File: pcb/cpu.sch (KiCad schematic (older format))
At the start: 28 parts, among them J100 Conn_02x05_Odd_Even, J101 Conn_02x05_Odd_Even, J102 Conn_02x05_Odd_Even, U100 MCIMX7S5EVM08SC, Y100 24MHz, Y101 32.768kHz

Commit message: pcb: remap schematic symbols
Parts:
- C100, C101, C102, C103, C104, C107, C108, C110: symbol pcb-rescue:C-Device-pcb-rescue -> Device:C
- D100: symbol pcb-rescue:D_Schottky-Device-pcb-rescue -> Device:D_Schottky
- J100, J101: symbol pcb-rescue:Conn_02x05_Odd_Even-Connector_Generic-pcb-rescue -> Connector_Generic:Conn_02x05_Odd_Even
- J102: symbol pcb-rescue:Conn_01x06-Connector_Generic-pcb-rescue -> Connector_Generic:Conn_01x06
- R102, R103, R104, R105, R106, R107, R108, R109, R110, R111: symbol pcb-rescue:R-Device-pcb-rescue -> Device:R
- RN100, RN101, RN102: symbol pcb-rescue:R_Pack04-Device-pcb-rescue -> Device:R_Pack04
- Y100: symbol pcb-rescue:Crystal_GND24-Device-pcb-rescue -> Device:Crystal_GND24
- Y101: symbol pcb-rescue:Crystal-Device-pcb-rescue -> Device:Crystal
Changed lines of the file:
@@
 	1700 1550 1900 1550
 $Comp
-L pcb-rescue:GND-power-pcb-rescue #PWR0101
+L power:GND #PWR0101
 U 1 1 5D1AEC8A
 P 1800 2050
@@
 	1900 2050 1800 2050
 $Comp
-L pcb-rescue:GND-power-pcb-rescue #PWR0102
+L power:GND #PWR0102
 U 1 1 5D1B0DA3
 P 3600 2950
@@
 NoConn ~ 3500 2350
 $Comp
-L pcb-rescue:C-Device-pcb-rescue C100
+L Device:C C100
 U 1 1 5D1B3DE6
 P 1800 3900
@@
 	1800 3750 1800 3650
 $Comp
-L pcb-rescue:GND-power-pcb-rescue #PWR0104
+L power:GND #PWR0104
 U 1 1 5D1B612A
 P 1800 4150
@@
 	1800 4050 1800 4150
 $Comp
-L pcb-rescue:Crystal-Device-pcb-rescue Y101
+L Device:Crystal Y101
 U 1 1 5D1B84E0
 P 5250 3750
@@
 $EndComp
 $Comp
-L pcb-rescue:Crystal_GND24-Device-pcb-rescue Y100
+L Device:Crystal_GND24 Y100
 U 1 1 5D1BAE47
 P 4350 4050
@@
 $EndComp
 $Comp
-L pcb-rescue:C-Device-pcb-rescue C101
+L Device:C C101
 U 1 1 5D1BC145
 P 5000 4000
@@
 $EndComp
 $Comp
-L pcb-rescue:C-Device-pcb-rescue C102
+L Device:C C102
 U 1 1 5D1BD063
 P 5500 4000
@@
 $EndComp
 $Comp
-L pcb-rescue:GND-power-pcb-rescue #PWR0105
+L power:GND #PWR0105
 U 1 1 5D1BD44D
 P 5000 4150
@@
 $EndComp
 $Comp
-L pcb-rescue:C-Device-pcb-rescue C103
+L Device:C C103
 U 1 1 5D1C36A2
 P 4100 4300
@@
 $EndComp
 $Comp
-L pcb-rescue:C-Device-pcb-rescue C104
+L Device:C C104
 U 1 1 5D1C36A8
 P 4600 4300
@@
 $EndComp
 $Comp
-L pcb-rescue:GND-power-pcb-rescue #PWR0106
+L power:GND #PWR0106
 U 1 1 5D1C36AE
 P 4100 4450
@@
 $EndComp
 $Comp
-L pcb-rescue:R-Device-pcb-rescue R102
+L Device:R R102
 U 1 1 5D1C3964
 P 4350 3650
@@
 $EndComp
 $Comp
-L pcb-rescue:R-Device-pcb-rescue R103
+L Device:R R103
 U 1 1 5D1C4735
 P 5250 3350
@@
 BT_CFG_14
 $Comp
-L pcb-rescue:R_Pack04-Device-pcb-rescue RN100
+L Device:R_Pack04 RN100
 U 1 1 5D1FE095
 P 1900 7100
@@
 $EndComp
 $Comp
-L pcb-rescue:R_Pack04-Device-pcb-rescue RN101
+L Device:R_Pack04 RN101
 U 1 1 5D2005B7
 P 2600 7100
@@
 $EndComp
 $Comp
-L pcb-rescue:R_Pack04-Device-pcb-rescue RN102
+L Device:R_Pack04 RN102
 U 1 1 5D206895
 P 1900 5300
@@
 	1800 6600 1800 6900
 $Comp
-L pcb-rescue:GND-power-pcb-rescue #PWR0107
+L power:GND #PWR0107
 U 1 1 5D21E58A
 P 1700 7300
@@
 $EndComp
 $Comp
-L pcb-rescue:+3V3-power-pcb-rescue #PWR0108
+L power:+3V3 #PWR0108
 U 1 1 5D21F0D5
 P 1700 5100
@@
 	2600 7300 2500 7300
 $Comp
-L pcb-rescue:R-Device-pcb-rescue R104
+L Device:R R104
 U 1 1 5D2235B5
 P 1000 1500
@@
 $EndComp
 $Comp
-L pcb-rescue:R-Device-pcb-rescue R105
+L Device:R R105
 U 1 1 5D2243E3
 P 1000 2100
@@
 $EndComp
 $Comp
-L pcb-rescue:R-Device-pcb-rescue R106
+L Device:R R106
 U 1 1 5D225B1C
 P 800 1500
@@
 $EndComp
 $Comp
-L pcb-rescue:R-Device-pcb-rescue R107
+L Device:R R107
 U 1 1 5D225B22
 P 800 2100
@@
 $EndComp
 $Comp
-L pcb-rescue:GND-power-pcb-rescue #PWR0109
+L power:GND #PWR0109
 U 1 1 5D227422
 P 1000 2450
@@
 NoConn ~ 1900 2750
 $Comp
-L pcb-rescue:GND-power-pcb-rescue #PWR0111
+L power:GND #PWR0111
 U 1 1 5D258935
 P 3600 2050
@@
 Connection ~ 1700 5100
 $Comp
-L pcb-rescue:Conn_02x05_Odd_Even-Connector_Generic-pcb-rescue J100
+L Connector_Generic:Conn_02x05_Odd_Even J100
 U 1 1 5D31C612
 P 7300 5900
@@
 $EndComp
 $Comp
-L pcb-rescue:+3V3-power-pcb-rescue #PWR0112
+L power:+3V3 #PWR0112
 U 1 1 5D32043C
 P 7000 5200
@@
 $EndComp
 $Comp
-L pcb-rescue:R-Device-pcb-rescue R108
+L Device:R R108
 U 1 1 5D32601B
 P 7700 5350
@@
 $EndComp
 $Comp
-L pcb-rescue:R-Device-pcb-rescue R109
+L Device:R R109
 U 1 1 5D327514
 P 8000 5350
@@
 Connection ~ 7000 5200
 $Comp
-L pcb-rescue:GND-power-pcb-rescue #PWR0113
+L power:GND #PWR0113
 U 1 1 5D35B6F4
 P 7000 6200
@@
 NoConn ~ 7100 6000
 $Comp
-L pcb-rescue:D_Schottky-Device-pcb-rescue D100
+L Device:D_Schottky D100
 U 1 1 5D37EF0D
 P 7950 6100
@@
 	9100 5500 9100 5700
 $Comp
-L pcb-rescue:+3V3-power-pcb-rescue #PWR0114
+L power:+3V3 #PWR0114
 U 1 1 5D3BDEDA
 P 9100 5500
@@
 $EndComp
 $Comp
-L pcb-rescue:GND-power-pcb-rescue #PWR0115
+L power:GND #PWR0115
 U 1 1 5D3BDA94
 P 9100 6200
@@
 CPLD JTAG
 $Comp
-L pcb-rescue:Conn_02x05_Odd_Even-Connector_Generic-pcb-rescue J101
+L Connector_Generic:Conn_02x05_Odd_Even J101
 U 1 1 5D31F9CC
 P 9400 5900
@@
 $EndComp
 $Comp
-L pcb-rescue:+3V3-power-pcb-rescue #PWR?
+L power:+3V3 #PWR?
 U 1 1 5D9DFFB8
 P 6600 1300
@@
 $EndComp
 $Comp
-L pcb-rescue:C-Device-pcb-rescue C?
+L Device:C C?
 U 1 1 5D9DFFBE
 P 6600 1650
@@
 $EndComp
 $Comp
-L pcb-rescue:GND-power-pcb-rescue #PWR?
+L power:GND #PWR?
 U 1 1 5D9DFFC4
 P 6600 1900
@@
 Connection ~ 6600 1300
 $Comp
-L pcb-rescue:+3V3-power-pcb-rescue #PWR?
+L power:+3V3 #PWR?
 U 1 1 5D9E5D3F
 P 6600 2500
@@
 $EndComp
 $Comp
-L pcb-rescue:C-Device-pcb-rescue C?
+L Device:C C?
 U 1 1 5D9E5D45
 P 6600 2850
@@
 $EndComp
 $Comp
-L pcb-rescue:GND-power-pcb-rescue #PWR?
+L power:GND #PWR?
 U 1 1 5D9E5D4B
 P 6600 3100
@@
 Connection ~ 6600 2500
 $Comp
-L pcb-rescue:+3V3-power-pcb-rescue #PWR?
+L power:+3V3 #PWR?
 U 1 1 5D9EC1DD
 P 6600 3500
@@
 $EndComp
 $Comp
-L pcb-rescue:C-Device-pcb-rescue C?
+L Device:C C?
 U 1 1 5D9F4B12
 P 6600 4250
@@
 	6600 4000 6600 4100
 $Comp
-L pcb-rescue:GND-power-pcb-rescue #PWR0122
+L power:GND #PWR0122
 U 1 1 5D9F4B1A
 P 6600 4400
@@
 	8400 1400 8650 1400
 $Comp
-L pcb-rescue:R-Device-pcb-rescue R110
+L Device:R R110
 U 1 1 5DA710EB
 P 8650 1050
@@
 $EndComp
 $Comp
-L pcb-rescue:R-Device-pcb-rescue R111
+L Device:R R111
 U 1 1 5DA7199D
 P 9050 1050
@@
 	8650 1200 8650 1400
 $Comp
-L pcb-rescue:+3V3-power-pcb-rescue #PWR?
+L power:+3V3 #PWR?
 U 1 1 5DA800C1
 P 8650 900
@@
 Connection ~ 8650 1400
 $Comp
-L pcb-rescue:Conn_01x06-Connector_Generic-pcb-rescue J102
+L Connector_Generic:Conn_01x06 J102
 U 1 1 5DA9BBD7
 P 10200 3400
@@
 	8400 3600 10000 3600
 $Comp
-L pcb-rescue:GND-power-pcb-rescue #PWR0124
+L power:GND #PWR0124
 U 1 1 5DAAF59A
 P 9900 3300

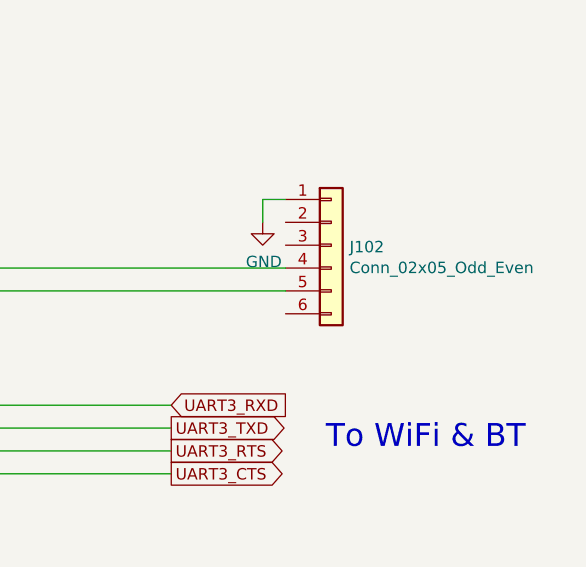
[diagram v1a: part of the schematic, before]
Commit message: pcb: bug fixes
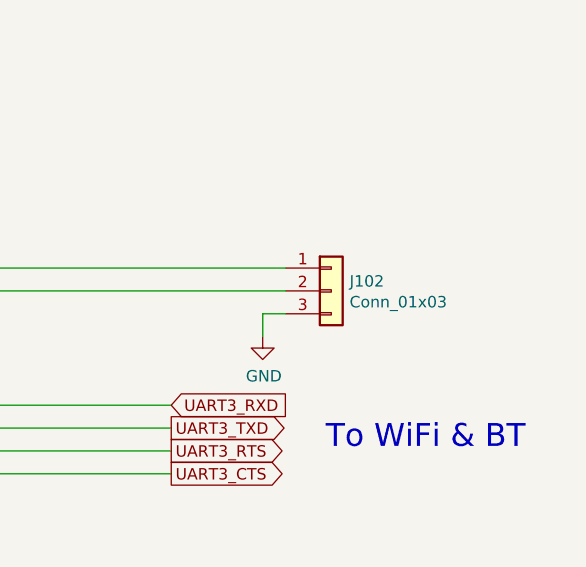
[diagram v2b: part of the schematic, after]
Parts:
- removed J102: Conn_02x05_Odd_Even, Connector_PinHeader_1.27mm:PinHeader_1x06_P1.27mm_Vertical, symbol Connector_Generic:Conn_01x06
- added J102: Conn_01x03, symbol Connector_Generic:Conn_01x03
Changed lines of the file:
@@
 	8650 1400 9500 1400
 Connection ~ 8650 1400
-$Comp
-L Connector_Generic:Conn_01x06 J102
-U 1 1 5DA9BBD7
-P 10200 3400
-F 0 "J102" H 10280 3392 50  0000 L CNN
-F 1 "Conn_02x05_Odd_Even" H 10280 3301 50  0000 L CNN
-F 2 "Connector_PinHeader_1.27mm:PinHeader_1x06_P1.27mm_Vertical" H 10200 3400 50  0001 C CNN
-F 3 "~" H 10200 3400 50  0001 C CNN
-	1    10200 3400
-	1    0    0    -1
-$EndComp
 Wire Wire Line
 	8400 3500 10000 3500
@@
 L power:GND #PWR0124
 U 1 1 5DAAF59A
-P 9900 3300
-F 0 "#PWR0124" H 9900 3050 50  0001 C CNN
-F 1 "GND" H 9905 3127 50  0000 C CNN
-F 2 "" H 9900 3300 50  0001 C CNN
-F 3 "" H 9900 3300 50  0001 C CNN
-	1    9900 3300
+P 9900 3800
+F 0 "#PWR0124" H 9900 3550 50  0001 C CNN
+F 1 "GND" H 9905 3627 50  0000 C CNN
+F 2 "" H 9900 3800 50  0001 C CNN
+F 3 "" H 9900 3800 50  0001 C CNN
+	1    9900 3800
 	1    0    0    -1
 $EndComp
 Wire Wire Line
-	10000 3200 9900 3200
+	10000 3700 9900 3700
 Wire Wire Line
-	9900 3200 9900 3300
+	9900 3700 9900 3800
 Text GLabel 9500 4100 2    50   Input ~ 0
 UART3_RXD
@@
 $EndComp
 Connection ~ 1000 1150
+$Comp
+L Connector_Generic:Conn_01x03 J102
+U 1 1 5D8590D0
+P 10200 3600
+F 0 "J102" H 10280 3642 50  0000 L CNN
+F 1 "Conn_01x03" H 10280 3551 50  0000 L CNN
+F 2 "" H 10200 3600 50  0001 C CNN
+F 3 "~" H 10200 3600 50  0001 C CNN
+	1    10200 3600
+	1    0    0    -1
+$EndComp
 $EndSCHEMATC

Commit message: fix #2
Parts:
- J102: footprint (none) -> Connector_PinHeader_2.54mm:PinHeader_1x03_P2.54mm_Vertical
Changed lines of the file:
@@
 F 0 "J102" H 10280 3642 50  0000 L CNN
 F 1 "Conn_01x03" H 10280 3551 50  0000 L CNN
-F 2 "" H 10200 3600 50  0001 C CNN
+F 2 "Connector_PinHeader_2.54mm:PinHeader_1x03_P2.54mm_Vertical" H 10200 3600 50  0001 C CNN
 F 3 "~" H 10200 3600 50  0001 C CNN
 	1    10200 3600
